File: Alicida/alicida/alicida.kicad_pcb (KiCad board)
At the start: 2 copper layers, 354.9 x 117.8 mm, 146 parts, among them SW1 SW_PUSH, U1 ATMEGA32U4, X1 XTAL_GND

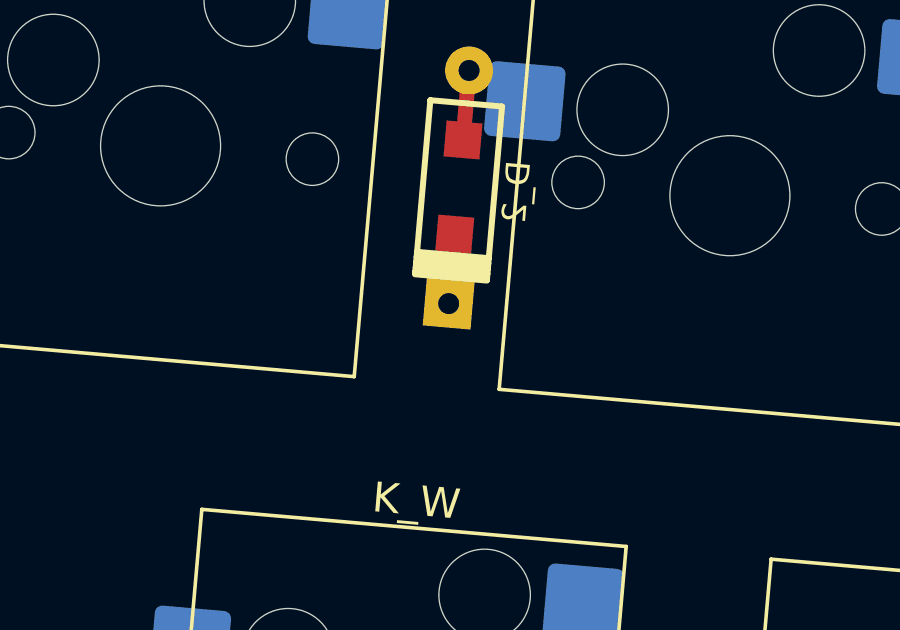
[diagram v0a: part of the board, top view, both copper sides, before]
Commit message: dfgh
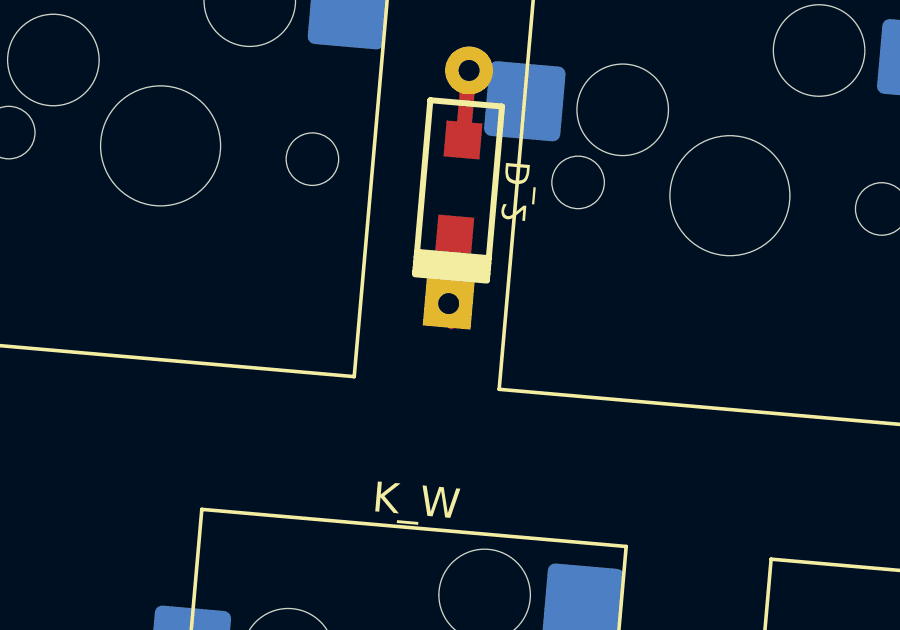
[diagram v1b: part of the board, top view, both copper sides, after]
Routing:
- net (no net): track 0.00 -> 0.80 mm
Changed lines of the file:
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@@
     (effects (font (size 1 1) (thickness 0.3)) (justify right))
   )
+  (segment (start 194.222484 173.84911) (end 194.222484 174.522484) (width 0.2) (layer "F.Cu") (net 0))
+  (segment (start 194.222484 174.522484) (end 194.31 174.61) (width 0.2) (layer "F.Cu") (net 0))
   (zone (net 0) (net_name "") (layer "F.Cu") (hatch edge 0.508)
     (connect_pads yes (clearance 0.25))

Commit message: update
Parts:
- added REF**: USB_C_Receptacle_Palconn_UTC16-G, Connector_USB:USB_C_Receptacle_Palconn_UTC16-G, F.Cu at (263.3, 153.4)
- added REF**: diode smd tht, keyboard_parts:diode smd tht, F.Cu at (150.9, 223.1)
- added REF**: diode smd tht, keyboard_parts:diode smd tht, F.Cu at (165.4, 242.0)
- added REF**: diode smd tht, keyboard_parts:diode smd tht, F.Cu at (423.2, 204.7)
- added REF**: diode smd tht, keyboard_parts:diode smd tht, F.Cu at (197.5, 246.2)
- added REF**: diode smd tht, keyboard_parts:diode smd tht, F.Cu at (361.9, 244.1)
- added REF**: diode smd tht, keyboard_parts:diode smd tht, F.Cu at (238.0, 250.1)
- added REF**: diode smd tht, keyboard_parts:diode smd tht, F.Cu at (144.0, 184.8)
- added REF**: diode smd tht, keyboard_parts:diode smd tht, F.Cu at (146.4, 203.8)
- added REF**: diode smd tht, keyboard_parts:diode smd tht, F.Cu at (394.8, 223.6)
- added REF**: diode smd tht, keyboard_parts:diode smd tht, F.Cu at (430.5, 185.6)
- added REF**: diode smd tht, keyboard_parts:diode smd tht, F.Cu at (425.6, 166.6)
- added REF**: diode smd tht, keyboard_parts:diode smd tht, F.Cu at (141.6, 241.9)
- added REF**: diode smd tht, keyboard_parts:diode smd tht, F.Cu at (321.4, 247.9)
- D_0, D_1, D_2, D_3, D_4, D_5, D_6, D_7, D_8, D_9, D_A, D_ALT, D_ALT1, D_B, D_BACKSPACE, D_BSLSH, D_C, D_CAPS, D_CBRAC, D_COMMA, D_CTRL, D_D, D_DOT, D_DOWN, D_E, D_ENTER, D_EQUAL, D_F, D_G, D_H, D_I, D_J, D_K, D_L, D_LEFT, D_M, D_MINUS, D_N, D_O, D_OBRAC, D_P, D_Q, D_QUOTE, D_R, D_RIGHT, D_S, D_SEMIC, D_SHIFT, D_SHIFT1, D_SLASH, D_SPACE, D_T, D_TAB, D_U, D_UP, D_V, D_W, D_WIN, D_X, D_Y, D_Z, D_`: footprint keyboard_parts:D_SOD123_axial -> keyboard_parts:nothing
- K_0, K_1, K_2, K_3, K_4, K_5, K_6, K_7, K_8, K_9, K_A, K_B, K_C, K_CBRAC, K_COMMA, K_D, K_DOT, K_DOWN, K_E, K_EQUAL, K_F, K_G, K_H, K_I, K_J, K_K, K_L, K_LEFT, K_M, K_MINUS, K_N, K_O, K_OBRAC, K_P, K_Q, K_QUOTE, K_R, K_RIGHT, K_S, K_SEMIC, K_T, K_U, K_UP, K_V, K_W, K_X, K_Y, K_Z, K_`: footprint Switch_Keyboard_Hotswap_Kailh:SW_Hotswap_Kailh_MX_1.00u -> keyboard_parts:hotswap mx with diode
- moved D_T 4.69 mm to (261.0, 190.4), turned to 80 degrees
- moved D_SLASH 4.68 mm to (261.2, 248.4), turned to 95 degrees
- moved D_B 4.46 mm to (272.2, 229.9), turned to 90 degrees
- moved D_L 3.79 mm to (356.0, 201.4), turned to 95 degrees
- moved D_3 0.19 mm to (213.6, 171.8)
- moved D_4 0.19 mm to (232.6, 173.5)
- moved K_3 0.19 mm to (203.7, 170.4)
- moved K_5 0.19 mm to (241.6, 173.7)
- moved REF** 0.19 mm to (230.3, 249.4)
- moved K_4 0.19 mm to (222.6, 172.1)
- moved D_2 0.19 mm to (194.6, 170.1)
- moved D_C 0.19 mm to (232.4, 230.8)
- moved D_E 0.19 mm to (221.4, 191.6)
- moved D_R 0.19 mm to (240.4, 193.3)
- moved D_V 0.19 mm to (251.3, 232.5)
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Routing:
- net (no net): track 0.80 -> 2752.4 mm
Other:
- board size 354.9 x 117.8 mm -> 362.9 x 120.4 mm
